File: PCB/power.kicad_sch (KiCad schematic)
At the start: 12 parts, among them U2 MAX20029ATIA/V+

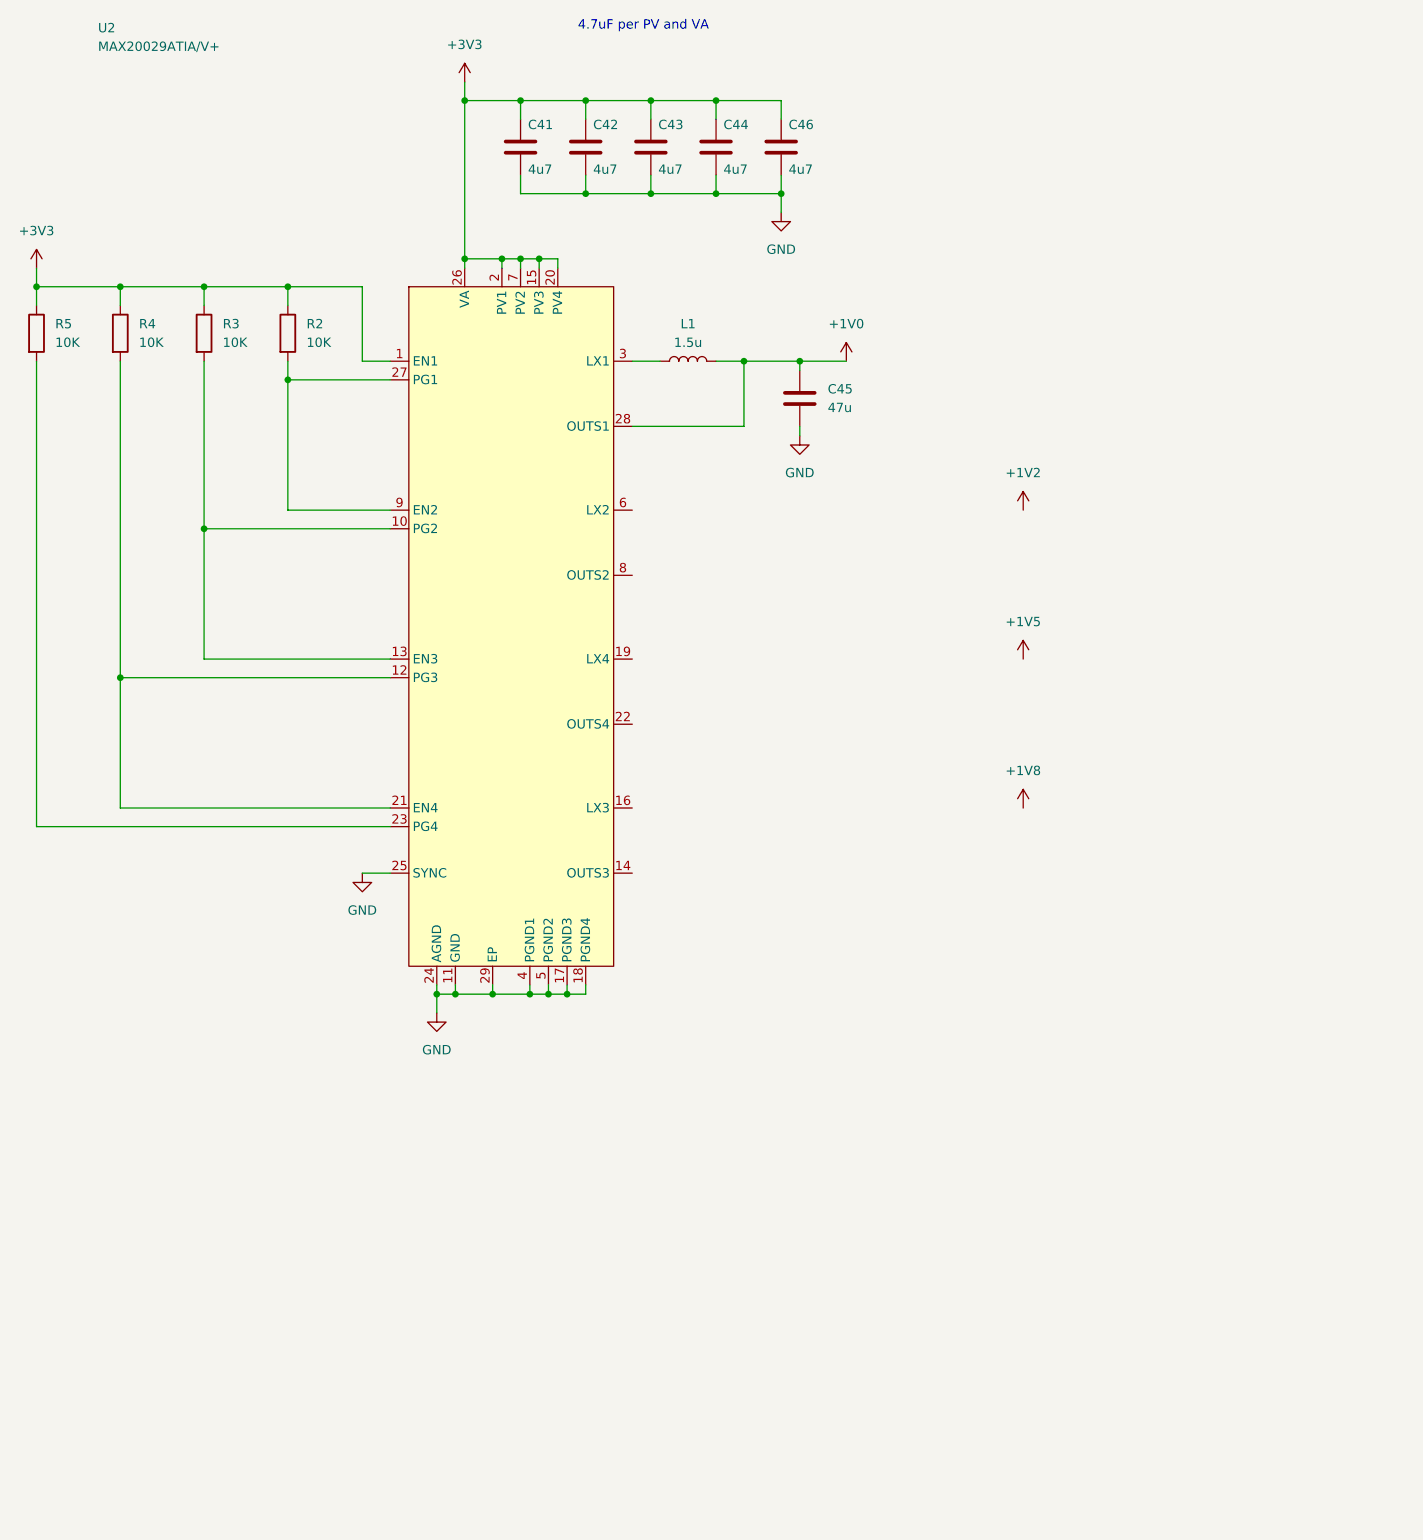
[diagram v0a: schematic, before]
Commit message: basic wiring finished
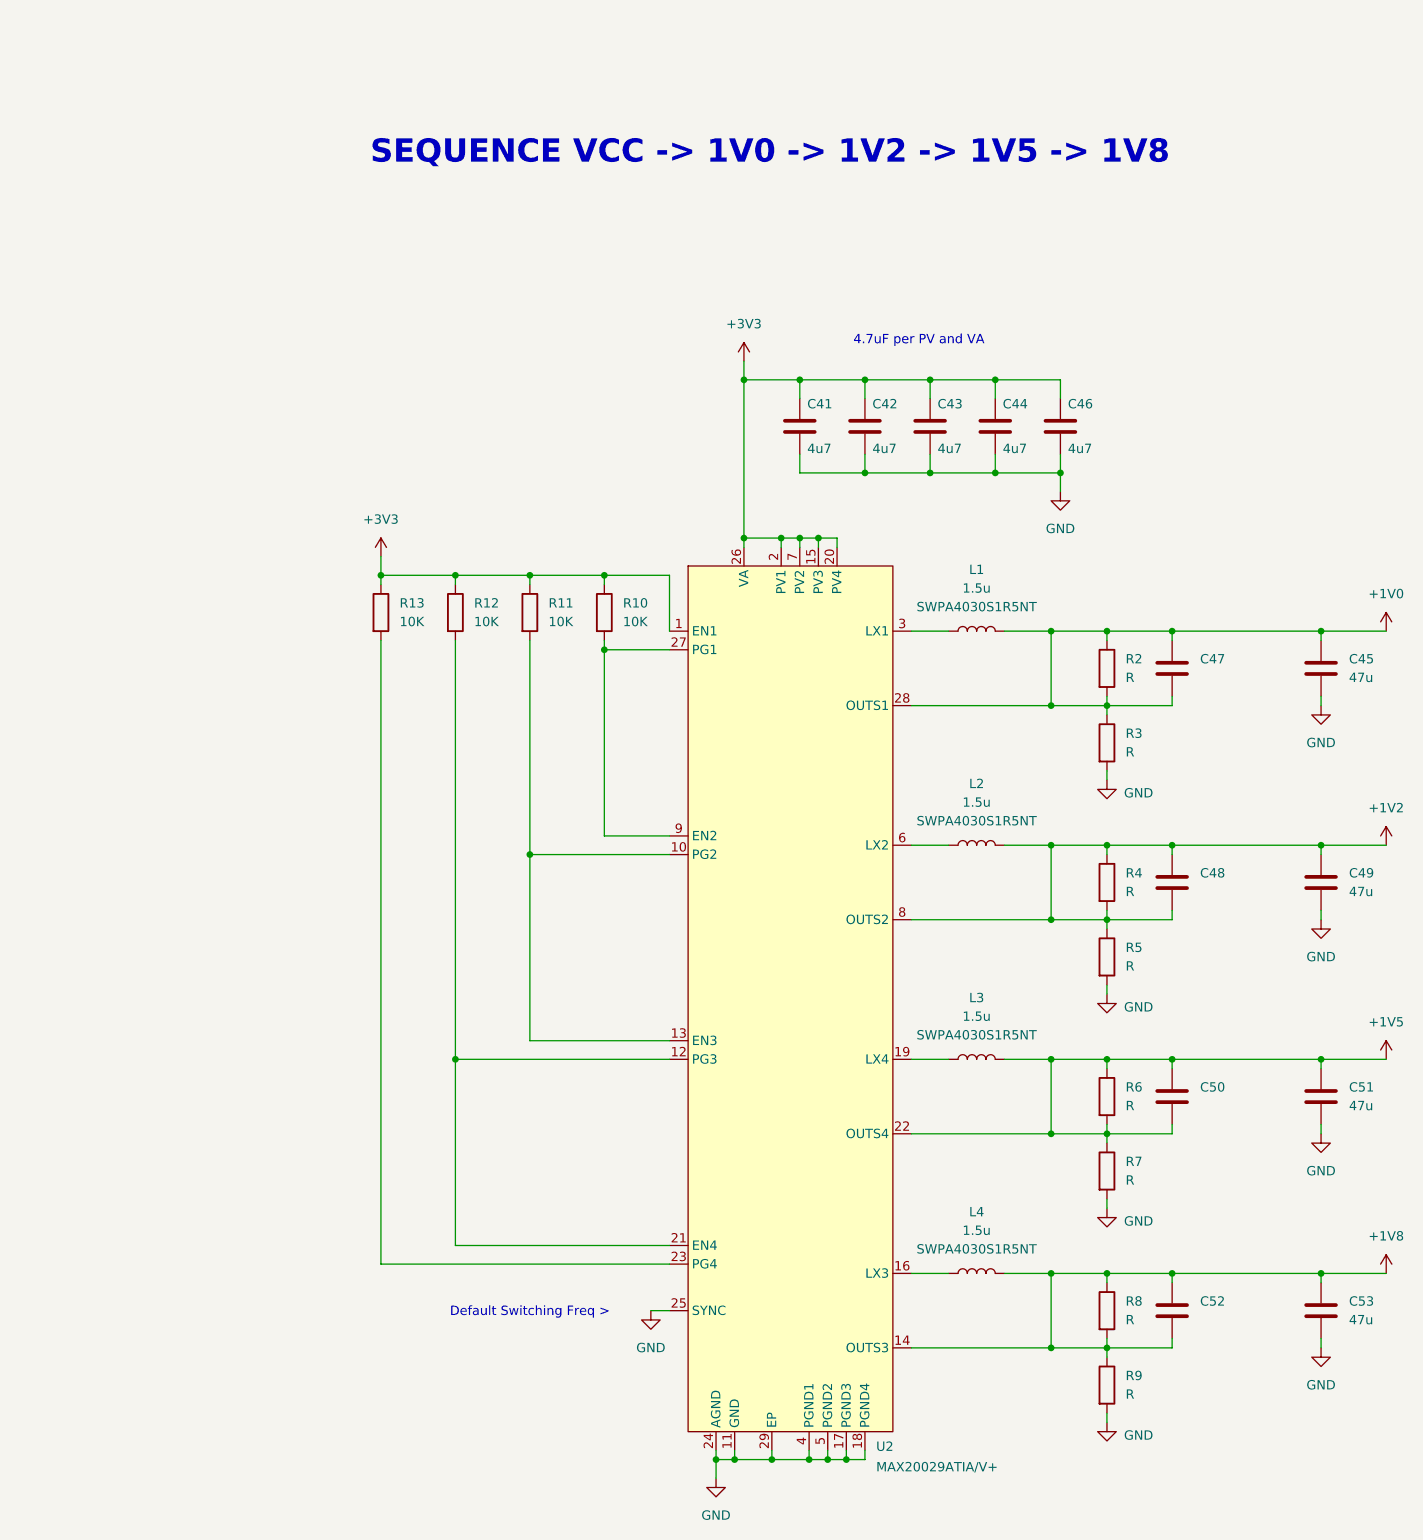
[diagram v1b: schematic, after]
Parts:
- added C47, C48, C50, C52: ~, symbol Device:C
- added C49, C51, C53: 47u, symbol Device:C
- added L2, L3, L4: 1.5u, symbol Device:L
- added R10, R11, R12, R13: 10K, symbol Device:R
- added R6, R7, R8, R9: R, symbol Device:R
- L1: LCSC (none) -> C42100; MPN (none) -> SWPA4030S1R5NT
- R2, R3, R4, R5: value 10K -> R
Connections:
- net +1V0: now also R2.1, R2.2, R3.1, C47.1, C47.2
- net +1V2: now also R4.1, R4.2, R5.1, U2.8 (OUTS2), C48.1, C48.2, C49.1, L2.2
- net +1V5: now also U2.22 (OUTS4), C50.1, C50.2, C51.1, L3.2, R6.1, R6.2, R7.1
- net +1V8: now also U2.14 (OUTS3), C52.1, C52.2, C53.1, L4.2, R8.1, R8.2, R9.1
- net +3V3: now also R10.1, R11.1, R12.1, R13.1; no longer R2.1, R3.1, R4.1, R5.1
- net GND: now also R3.2, R5.2, C49.2, C51.2, C53.2, R7.2, R9.2
- net at U2.27 (PG1), U2.9 (EN2): now also R10.2; no longer R2.2
- net at U2.10 (PG2), U2.13 (EN3): now also R11.2; no longer R3.2
- net at U2.12 (PG3), U2.21 (EN4): now also R12.2; no longer R4.2
- net at U2.16 (LX3): now also L4.1
- net at U2.19 (LX4): now also L3.1
- net at U2.23 (PG4): now also R13.2; no longer R5.2
- net at U2.6 (LX2): now also L2.1
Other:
- note added: "Default Switching Freq >"
- note added: "SEQUENCE VCC -> 1V0 -> 1V2 -> 1V5 -> 1V8"
- moved on the sheet: C41, C42, C43, C44, C45, C46, L1, U2
